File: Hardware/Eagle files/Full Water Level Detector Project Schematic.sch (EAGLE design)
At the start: 23 parts, among them IC1 74AHCT125, M1 SMALL_SERVO

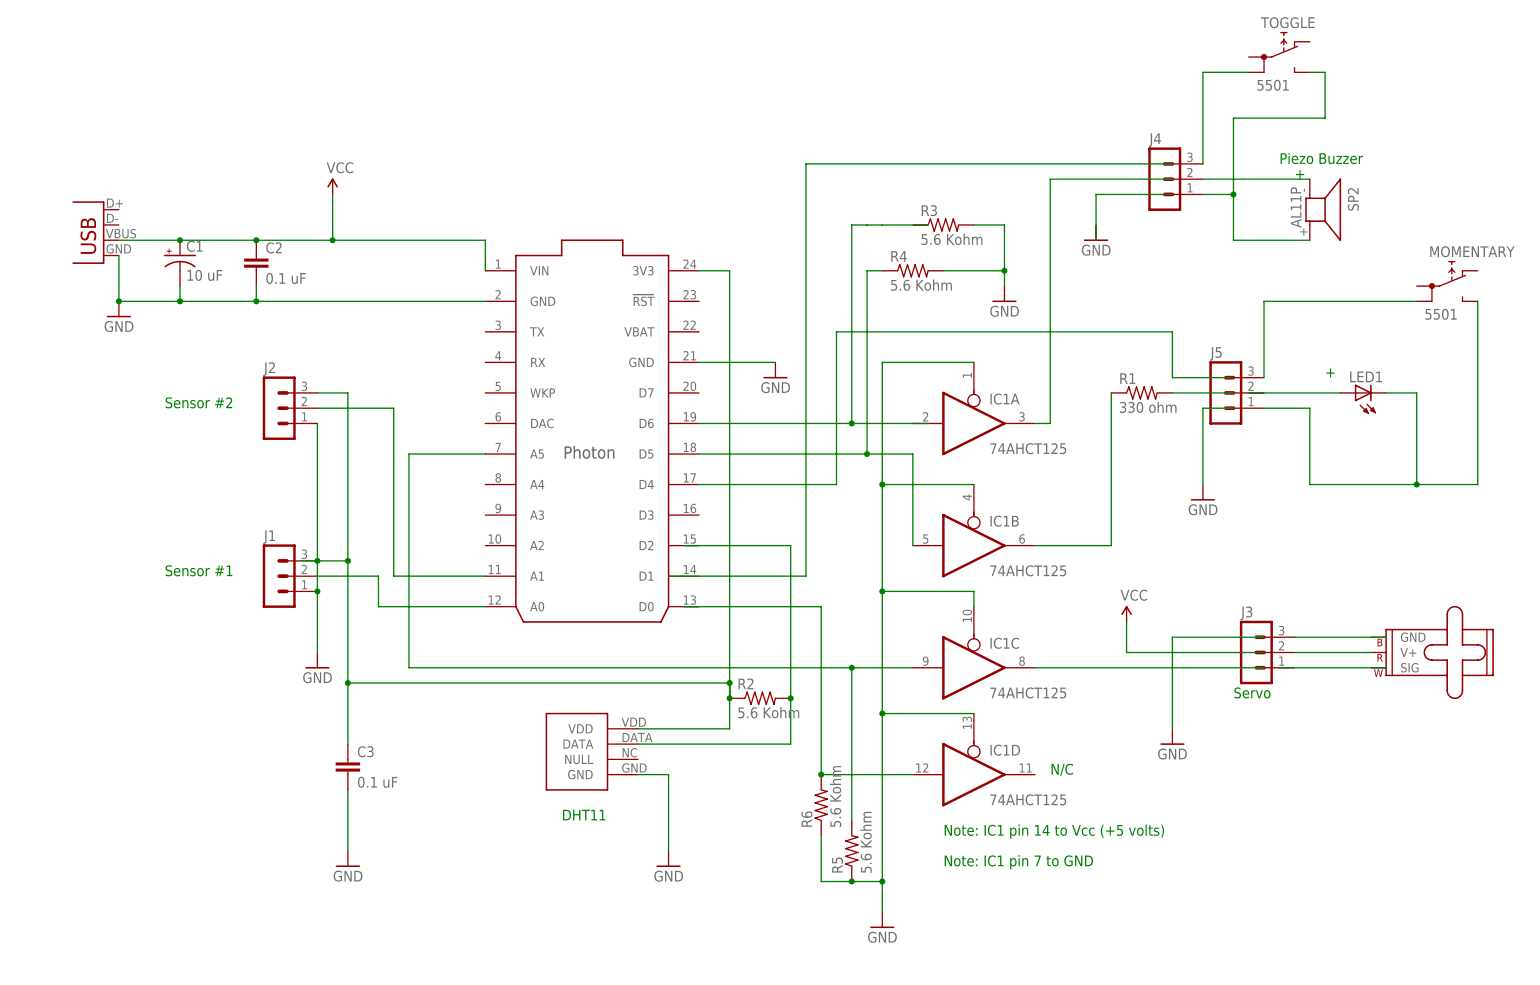
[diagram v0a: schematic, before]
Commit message: Final PCB Eagle Files
Final copies of Eagle schematic and board files as well as PDFs of
these.
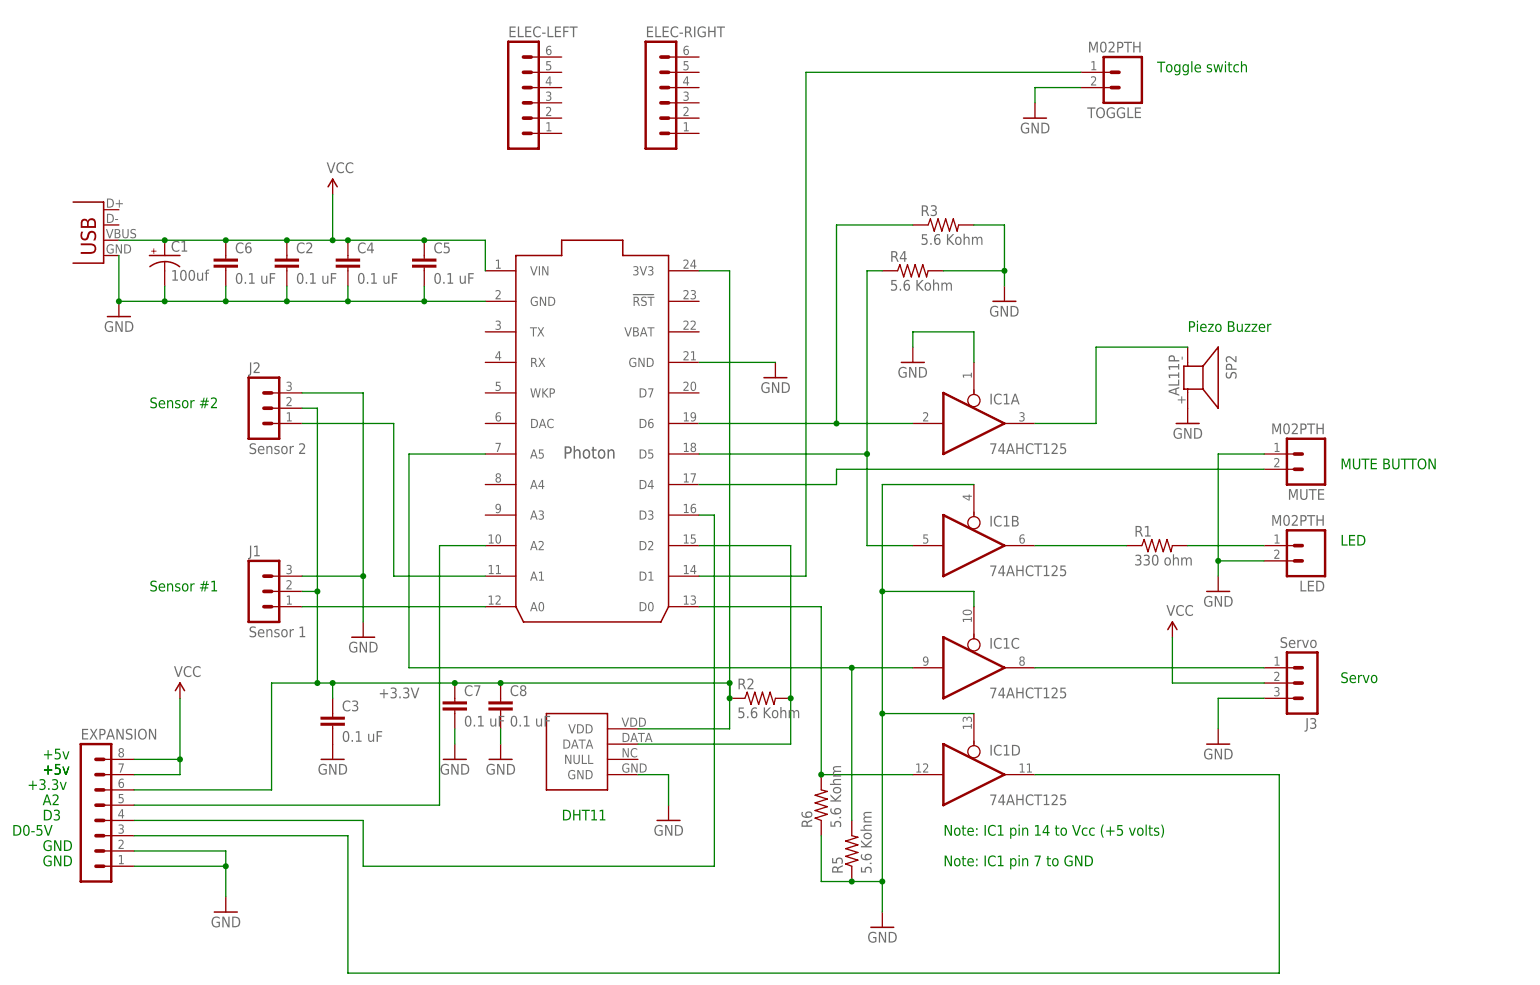
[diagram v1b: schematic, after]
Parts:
- removed J4, J5: (no value), con-lstb:MA03-1
- removed LED1: (no value), led:LED5MM
- removed M1: SMALL_SERVO, SparkFun-Electromechanical:SMALL_SERVO
- removed MOMENTARY: 5501, switch:5501
- added C4, C5, C6, C7, C8: 0.1 uF, SparkFun-Passives:CAPPTH
- added ELEC-LEFT, ELEC-RIGHT: (no value), con-lstb:MA06-1
- added EXPANSION: (no value), con-lstb:MA08-1
- added LED, MUTE: M02PTH, SparkFun-Connectors:M02PTH
- C1: value 10 uF -> 100uf; device SparkFun-Passives:CAP_POLPTH2 -> SparkFun-Capacitors:CAP_POLPTH1
- J1: value (none) -> Sensor 1
- J2: value (none) -> Sensor 2
- J3: value (none) -> Servo
- TOGGLE: value 5501 -> M02PTH; device switch:5501 -> SparkFun-Connectors:M02PTH
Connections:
- removed net N$12: U$1G$1.D4
- removed net N$13: IC1A.O
- removed net N$20: IC1C.O
- removed net N$21: J4.3, TOGGLE.1B
- removed net N$24: J5.3, MOMENTARY.1B
- removed net N$5: U$1G$1.D6
- removed net N$8: C3.1, J1.3, J2.3, R2.1, U$1G$1.3V3, U$2.VDD
- new net +3.3V: C3.1, C7.1, C8.1, EXPANSION.6, J1.2, J2.2, R2.1, U$1G$1.3V3, U$2.VDD
- new net N$16: EXPANSION.5, U$1G$1.A2
- new net N$6: IC1A.O, SP2.1
- net GND: now also C4.2, C5.2, C6.2, C7.2, C8.2, EXPANSION.1, EXPANSION.2, J1.3, J2.3, J3.3, LED.2, MUTE.1, SP2.2, TOGGLE.2; no longer J1.1, J2.1
- net N$1: now also IC1C.O, J3.1; no longer J3.3
- net N$10: now also LED.1, R1.2; no longer J5.1, LED1.C, MOMENTARY.NO
- net N$11: now also MUTE.2, U$1G$1.D4; no longer J4.2, SP2.1
- net N$14: now also EXPANSION.4, U$1G$1.D3; no longer J4.1, SP2.2, TOGGLE.NO
- net N$15: now also EXPANSION.3, IC1D.O; no longer R1.2
- net N$17: now also U$1G$1.D0
- net N$19: now also U$1G$1.D2
- net N$2: now also J2.1, U$1G$1.A1; no longer J1.2, U$1G$1.A0
- net N$22: now also TOGGLE.1, U$1G$1.D1; no longer LED1.A
- net N$3: now also J1.1, U$1G$1.A0; no longer J2.2, U$1G$1.A1
- net N$4: now also IC1A.I, R3.1, U$1G$1.D6; no longer J3.2, M1.V+
- net VCC: now also C4.1, C5.1, C6.1, EXPANSION.7, EXPANSION.8, J3.2
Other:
- note added: "+3.3v"
- note added: "+5v"
- note added: "A2"
- note added: "D0-5V"
- note added: "D3"
- note added: "GND"
- note added: "LED"
- note added: "MUTE BUTTON"
- note added: "Toggle switch"
- note removed: "+"
- note removed: "N/C"
- moved on the sheet: C1, C2, C3, J1, J2, J3, R1, SP2
